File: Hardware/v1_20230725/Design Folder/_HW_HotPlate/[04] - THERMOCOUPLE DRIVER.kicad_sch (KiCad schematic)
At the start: 10 parts, among them J401 RECEPT_2X1_VERT_2.54MM, U401 MAX31855JASA+T

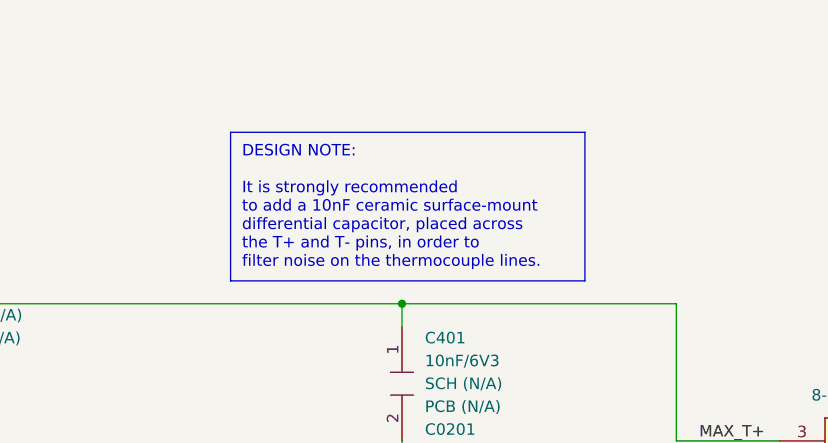
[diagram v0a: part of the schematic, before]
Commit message: Updating hardware format structure
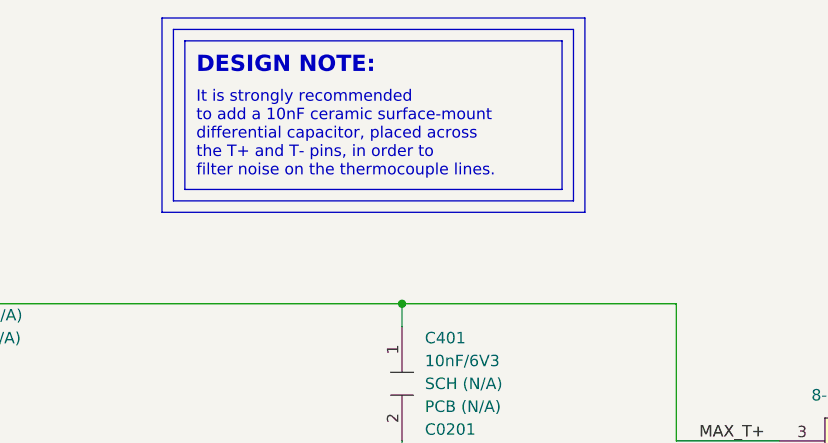
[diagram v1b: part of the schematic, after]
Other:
- note added: "DESIGN NOTE:"
- note added: "It is strongly recommended to add a 10nF ceramic surface-mount differential capacitor, placed across the T+ and T- pins, in order to filter noise on the thermocouple lines."
- note removed: "DESIGN NOTE: It is strongly recommended to add a 10nF ceramic surface-mount differential capacitor, placed across the T+ and T- pins, in order to filter noise on the thermocouple lines."
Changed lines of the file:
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@@
+    (stroke (width 0) (type default))
+  )
+  (polyline (pts (xy 189.23 125.73) (xy 189.23 144.78))
     (stroke (width 0) (type default))
   )
@@
   )
   (wire (pts (xy 236.22 176.53) (xy 236.22 177.8))
+    (stroke (width 0) (type default))
+  )
+  (polyline (pts (xy 187.96 124.46) (xy 187.96 146.05))
+    (stroke (width 0) (type default))
+  )
+  (polyline (pts (xy 234.95 124.46) (xy 234.95 146.05))
     (stroke (width 0) (type default))
   )
@@
     (stroke (width 0) (type default))
   )
+  (polyline (pts (xy 233.68 125.73) (xy 233.68 144.78))
+    (stroke (width 0) (type default))
+  )
+  (polyline (pts (xy 189.23 125.73) (xy 233.68 125.73))
+    (stroke (width 0) (type default))
+  )
   (wire (pts (xy 214.63 191.77) (xy 236.22 191.77))
     (stroke (width 0) (type default))
@@
   )
   (wire (pts (xy 284.48 176.53) (xy 334.01 176.53))
+    (stroke (width 0) (type default))
+  )
+  (polyline (pts (xy 187.96 146.05) (xy 234.95 146.05))
     (stroke (width 0) (type default))
   )
@@
     (stroke (width 0) (type default))
   )
+  (polyline (pts (xy 187.96 124.46) (xy 234.95 124.46))
+    (stroke (width 0) (type default))
+  )
   (wire (pts (xy 236.22 191.77) (xy 255.27 191.77))
     (stroke (width 0) (type default))
@@
     (stroke (width 0) (type default))
   )
+  (polyline (pts (xy 233.68 144.78) (xy 189.23 144.78))
+    (stroke (width 0) (type default))
+  )
   (wire (pts (xy 236.22 190.5) (xy 236.22 191.77))
     (stroke (width 0) (type default))
   )
-  (rectangle (start 195.58 137.16) (end 234.95 153.67)
+  (rectangle (start 190.5 127) (end 232.41 143.51)
     (stroke (width 0) (type default))
     (fill (type none))
+  )
+  (text "DESIGN NOTE:" (at 191.77 130.81 0)
+    (effects (font (size 1.8 1.8) bold) (justify left bottom))
   )
   (text "I = 1.5mA @ +3V3DC" (at 189.23 180.34 0)
     (effects (font (size 1.27 1.27)) (justify left bottom))
   )
-  (text "DESIGN NOTE:\n\nIt is strongly recommended \nto add a 10nF ceramic surface-mount\ndifferential capacitor, placed across\nthe T+ and T- pins, in order to \nfilter noise on the thermocouple lines.\n"
-    (at 196.85 152.4 0)
+  (text "\nIt is strongly recommended \nto add a 10nF ceramic surface-mount\ndifferential capacitor, placed across\nthe T+ and T- pins, in order to \nfilter noise on the thermocouple lines.\n"
+    (at 191.77 142.24 0)
     (effects (font (size 1.27 1.27)) (justify left bottom))
   )
